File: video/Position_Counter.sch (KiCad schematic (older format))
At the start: 14 parts, among them U22 74LS04, U23 74LS163, U24 74LS163, U25 74LS163, U26 74LS04, U27 74LS83, U28 74LS83, U29 74LS32, U30 74LS83, U31 74LS20, U32 74LS08, U33 74LS163, U34 74LS163, U35 74LS163

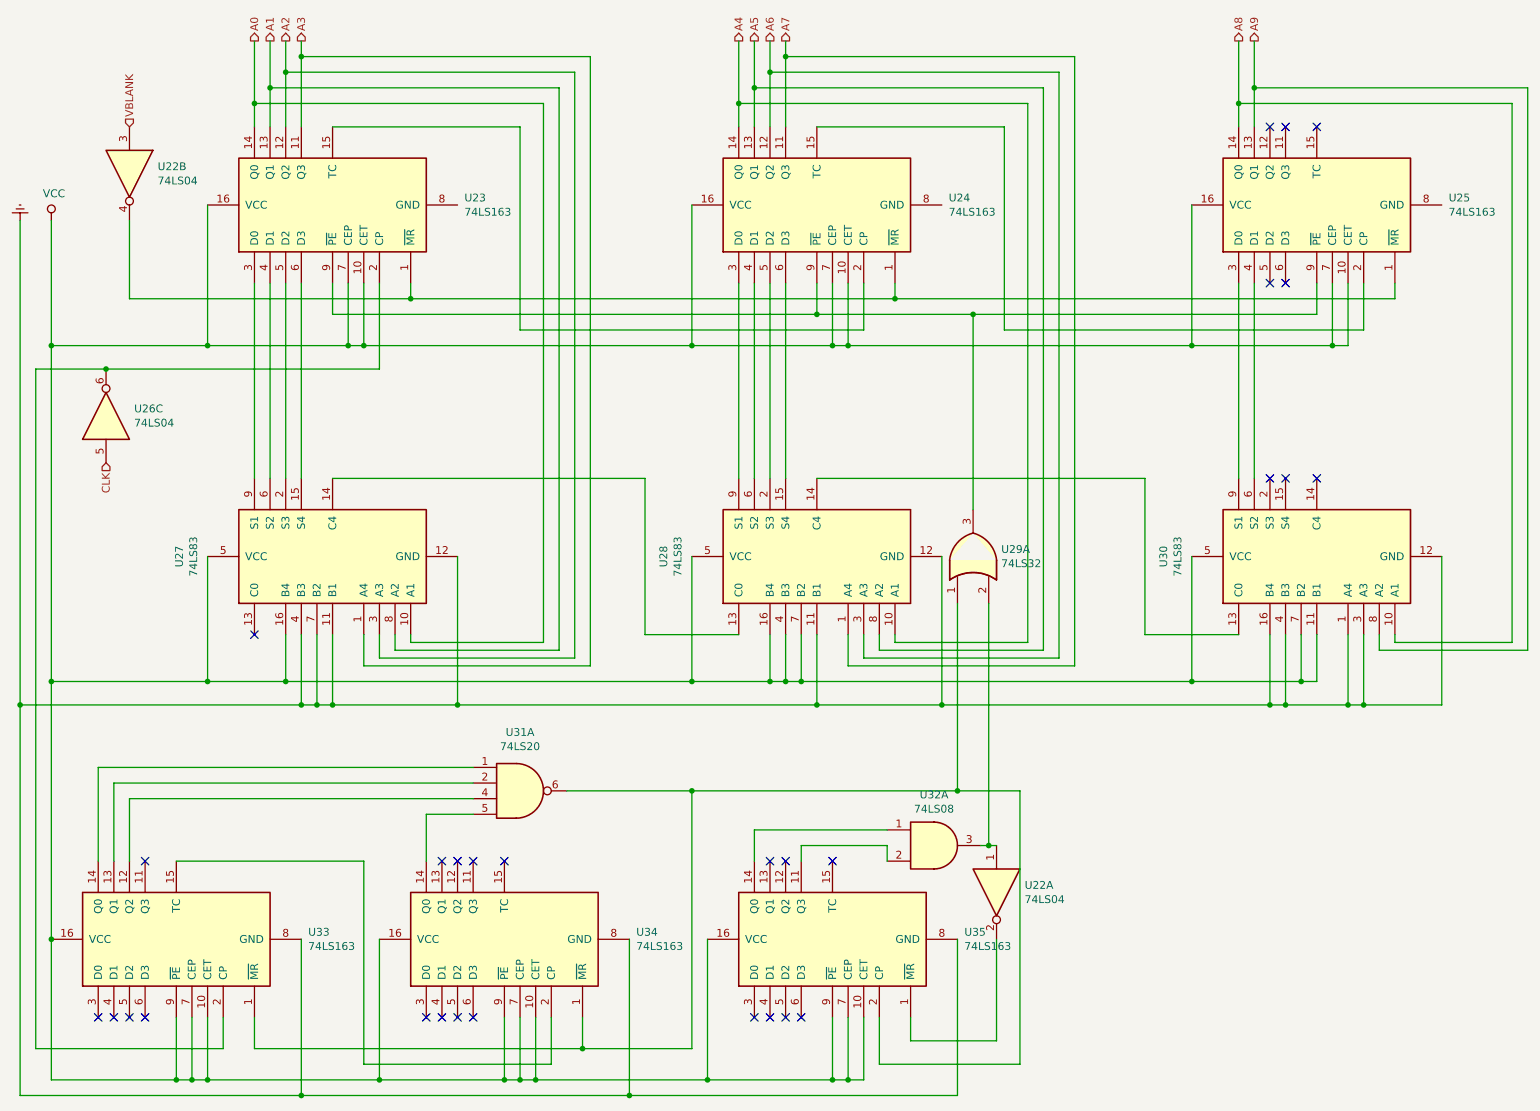
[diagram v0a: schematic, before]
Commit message: Resize and plot video
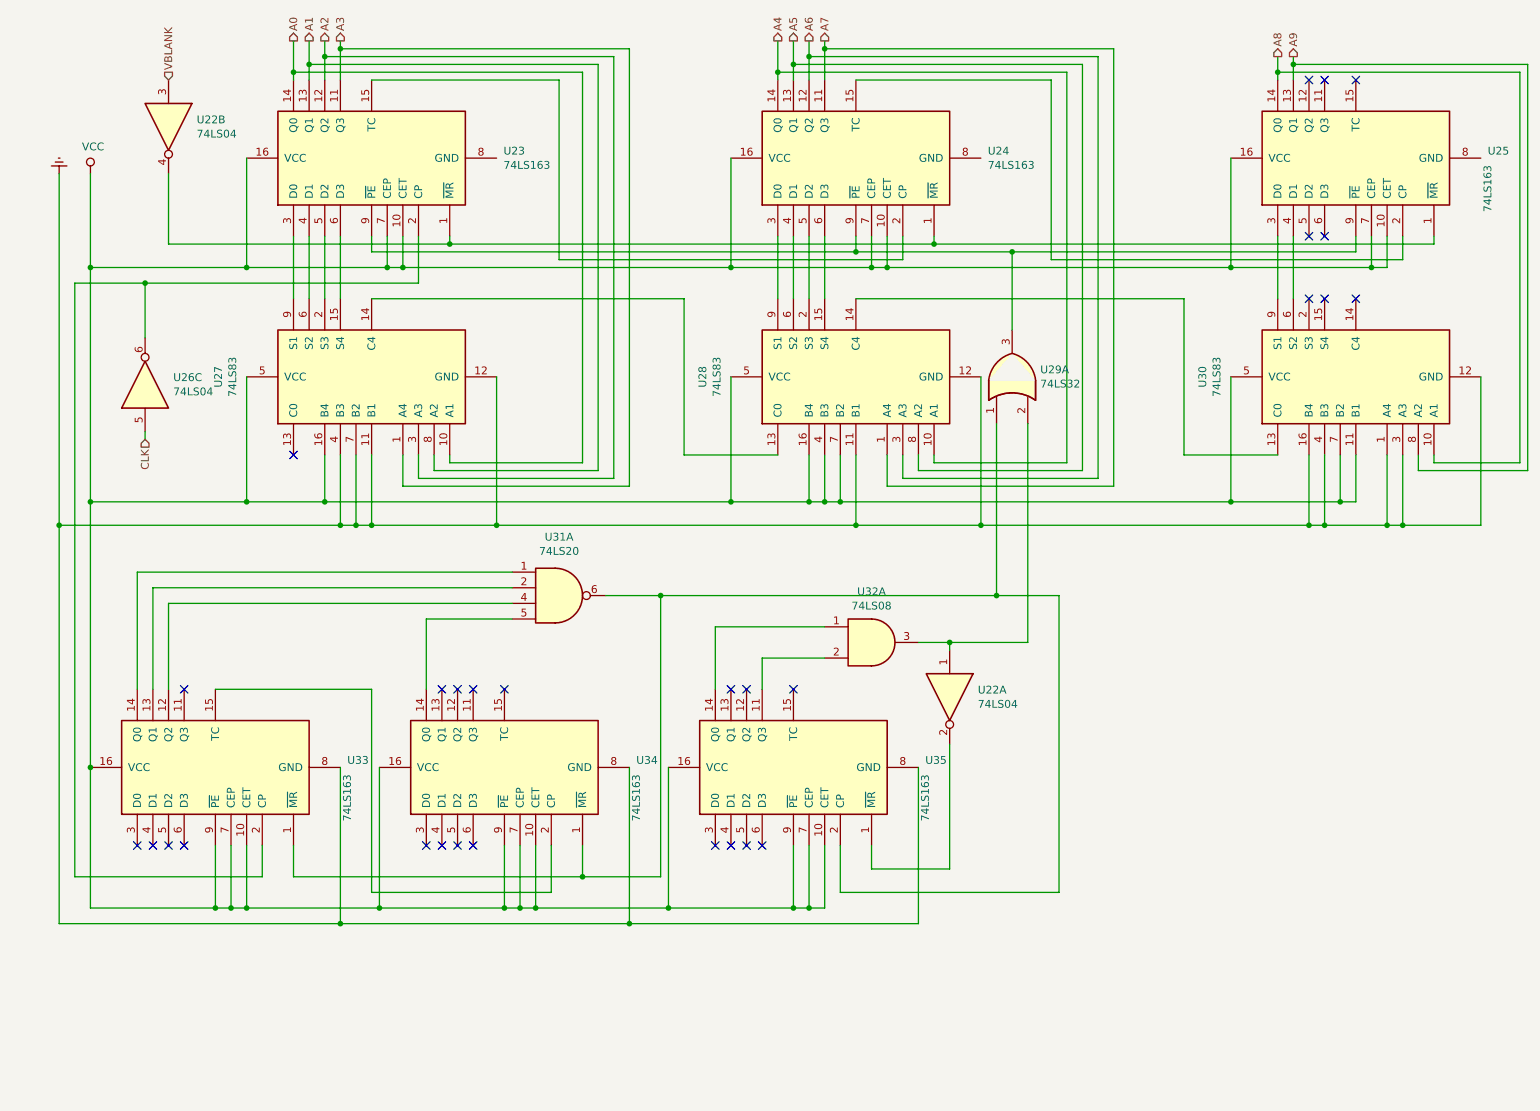
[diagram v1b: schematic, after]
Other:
- moved on the sheet: U22A, U22B, U23, U24, U25, U26C, U27, U28, U29A, U30, U31A, U32A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
